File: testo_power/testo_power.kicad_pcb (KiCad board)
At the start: 2 copper layers, 21 x 35 mm, 8 parts, among them J1 Conn_01x06_Pin, J2 Conn_01x02_Socket, J3 Conn_01x02_Socket, Q1 FQP27P06

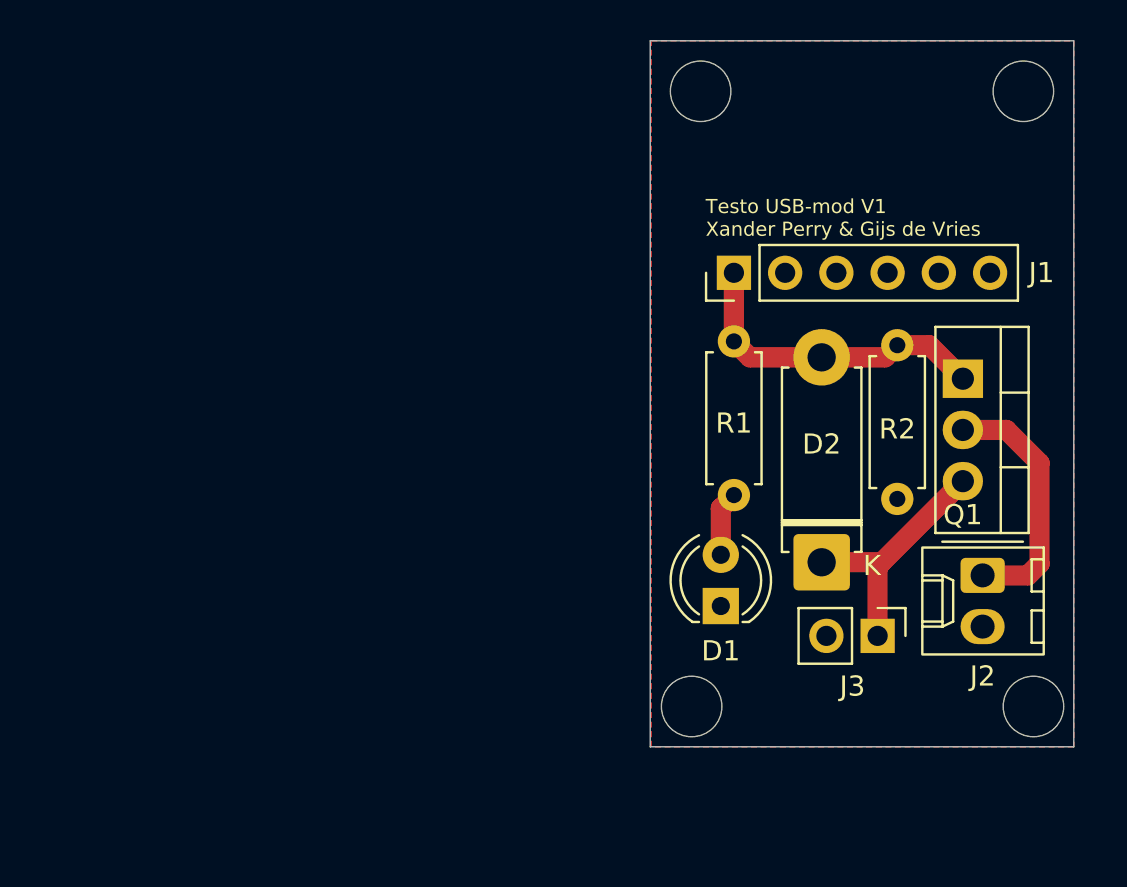
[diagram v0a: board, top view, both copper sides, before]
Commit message: pcb and schematic done
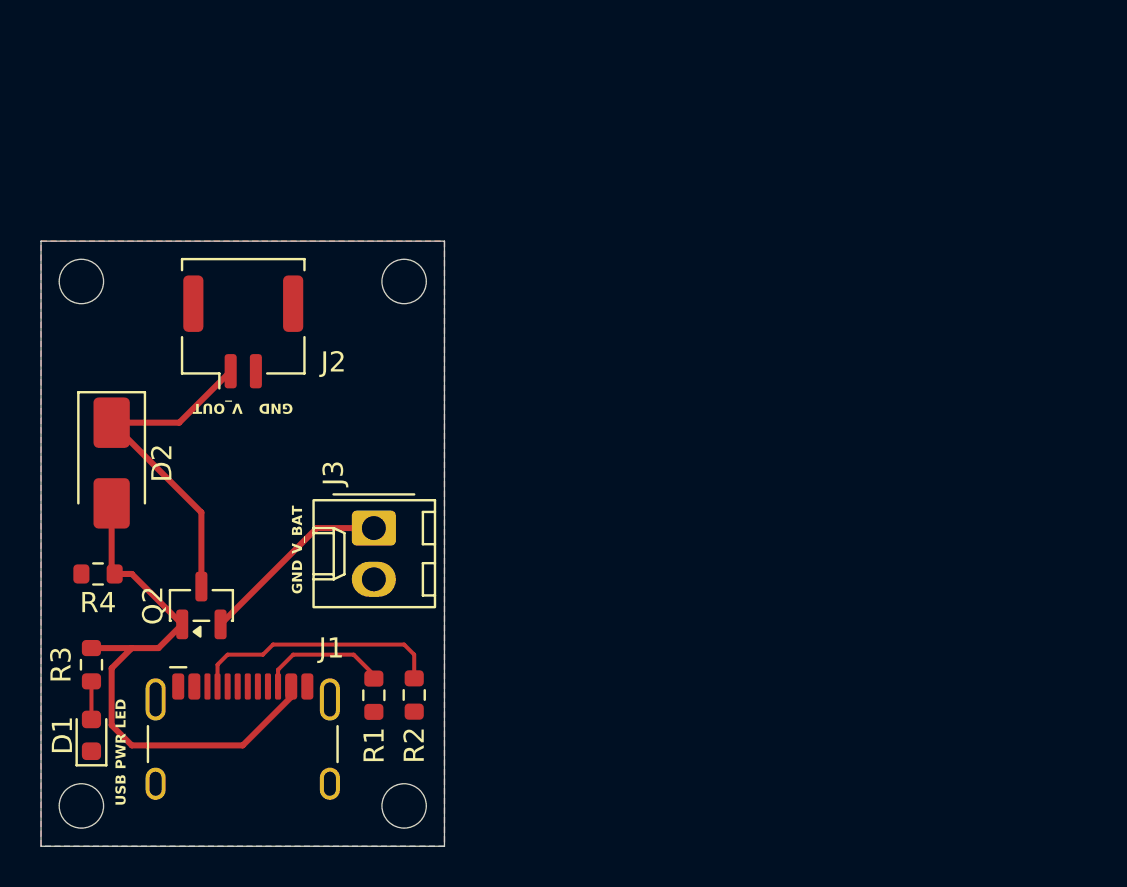
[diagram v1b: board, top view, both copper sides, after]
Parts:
- removed Q1: FQP27P06, Package_TO_SOT_THT:TO-220-3_Vertical
- added Q2: IRLML6402TRPBF, Package_TO_SOT_SMD:SOT-23, F.Cu at (108.0, 118.1)
- added R3: 150R, Resistor_SMD:R_0603_1608Metric, F.Cu at (102.5, 121.0)
- added R4: 10k, Resistor_SMD:R_0603_1608Metric, F.Cu at (102.8, 116.5)
- D1: value LED GRN -> LED RED; footprint LED_THT:LED_D4.0mm -> LED_SMD:LED_0603_1608Metric
- D2: value D_Schottky -> SS14; footprint Diode_THT:D_5W_P10.16mm_Horizontal -> Diode_SMD:D_SMA
- J1: value Conn_01x06_Pin -> USB_C_Receptacle_PowerOnly_6P; footprint Connector_PinHeader_2.54mm:PinHeader_1x06_P2.54mm_Vertical -> Connector_USB:USB_C_Receptacle_HCTL_HC-TYPE-C-16P-01A
- J2: footprint Connector_Molex:Molex_KK-254_AE-6410-02A_1x02_P2.54mm_Vertical -> Connector_Molex:Molex_CLIK-Mate_502382-0270_1x02-1MP_P1.25mm_Vertical
- J3: footprint Connector_PinHeader_2.54mm:PinHeader_1x02_P2.54mm_Vertical -> Connector_Molex:Molex_KK-254_AE-6410-02A_1x02_P2.54mm_Vertical
- R1: value 150 -> 5k1; footprint Resistor_THT:R_Axial_DIN0207_L6.3mm_D2.5mm_P7.62mm_Horizontal -> Resistor_SMD:R_0603_1608Metric
- R2: value 10k -> 5k1; footprint Resistor_THT:R_Axial_DIN0207_L6.3mm_D2.5mm_P7.62mm_Horizontal -> Resistor_SMD:R_0603_1608Metric
- moved J2 38.6 mm to (110.0, 104.5), turned to 0 degrees
- moved D2 35.5 mm to (103.5, 111.0), turned to -90 degrees
- moved J1 34.4 mm to (110.0, 125.8), turned to 0 degrees
- moved D1 31.9 mm to (102.5, 124.5)
- moved R2 29.6 mm to (118.5, 122.5), turned to 90 degrees
- moved J3 25.5 mm to (116.5, 114.2)
- moved R1 25.0 mm to (116.5, 122.5), turned to 90 degrees
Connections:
- D2 pad 2: V_USB -> V_BUS
- J2 pad 1: V_BAT -> V_OUT
- J3 pad 1: V_OUT -> V_BAT
- R1 pad 1: V_USB -> GND
- R1 pad 2: Net-(D1-A) -> Net-(J1-CC2)
- R2 pad 1: V_USB -> GND
- R2 pad 2: GND -> Net-(J1-CC1)
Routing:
- net V_BUS: track 0.00 -> 28.0 mm
- net V_USB: track 16.0 -> 0.00 mm
- net Net-(J1-CC1): track 0.00 -> 12.6 mm
- net Net-(J1-CC2): track 0.00 -> 6.49 mm
- net V_OUT: track 12.8 -> 16.9 mm
- net V_BAT: track 12.5 -> 9.58 mm
- net Net-(D1-A): track 3.23 -> 1.89 mm
- added copper zone on B.Cu, net GND
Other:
- board size 21 x 35 mm -> 20 x 30 mm
- board text added: "GND"
- board text added: "USB PWR LED"
- board text added: "V_BAT"
- board text added: "V_OUT"
- board text removed: "Testo USB-mod V1 Xander Perry & Gijs de Vries"
- board text removed: "USB-C breakout board"
